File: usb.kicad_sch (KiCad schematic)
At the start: 20 parts, among them J12 USB_A, J3 2169900003, Q1 MMBT3904, U12 STMPS2141STR

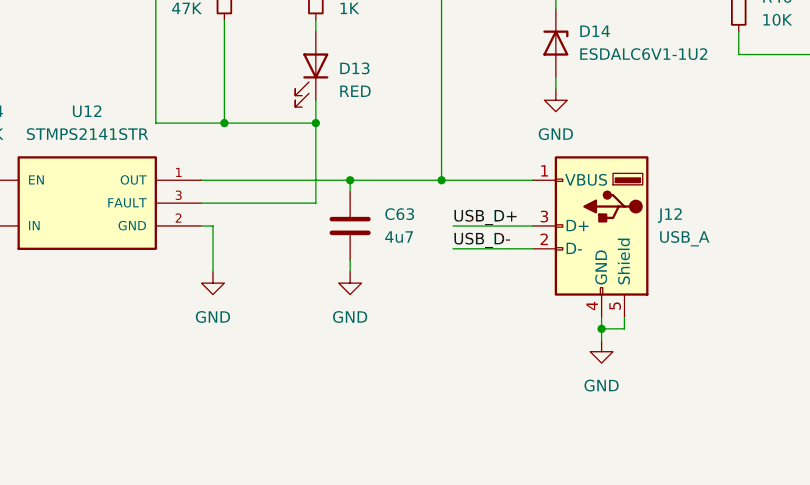
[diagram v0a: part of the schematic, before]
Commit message: First release
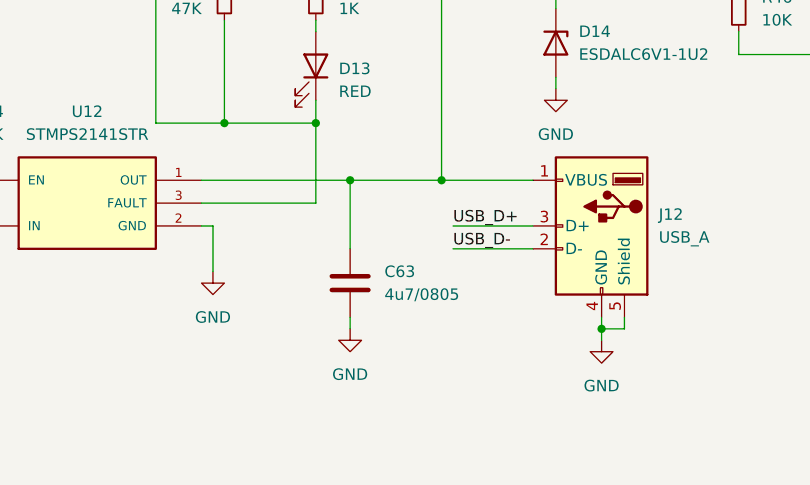
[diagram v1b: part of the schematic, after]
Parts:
- C63: value 4u7 -> 4u7/0805
- D14: JLCPCB Part # (none) -> C1974498; now left out of the parts list
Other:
- moved on the sheet: C63
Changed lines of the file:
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@@
 	(wire
 		(pts
-			(xy 109.22 121.92) (xy 109.22 123.19)
+			(xy 109.22 128.27) (xy 109.22 129.54)
 		)
 		(stroke
@@
 	(wire
 		(pts
-			(xy 109.22 113.03) (xy 109.22 114.3)
+			(xy 109.22 113.03) (xy 109.22 120.65)
 		)
 		(stroke
@@
 	(symbol
 		(lib_id "Device:C")
-		(at 109.22 118.11 0)
+		(at 109.22 124.46 0)
 		(unit 1)
 		(exclude_from_sim no)
@@
 		(fields_autoplaced yes)
 		(property "Reference" "C63"
-			(at 113.03 116.8399 0)
+			(at 113.03 123.1899 0)
 			(effects
 				(font
@@
 			)
 		)
-		(property "Value" "4u7"
-			(at 113.03 119.3799 0)
+		(property "Value" "4u7/0805"
+			(at 113.03 125.7299 0)
 			(effects
 				(font
@@
 		)
 		(property "Footprint" "Capacitor_SMD:C_0805_2012Metric"
-			(at 110.1852 121.92 0)
+			(at 110.1852 128.27 0)
 			(effects
 				(font
@@
 		)
 		(property "Datasheet" "~"
-			(at 109.22 118.11 0)
+			(at 109.22 124.46 0)
 			(effects
 				(font
@@
 		)
 		(property "Description" "Unpolarized capacitor"
-			(at 109.22 118.11 0)
+			(at 109.22 124.46 0)
 			(effects
 				(font
@@
 		)
 		(property "JLCPCB Part #" "C98192"
-			(at 109.22 118.11 0)
+			(at 109.22 124.46 0)
 			(effects
 				(font
@@
 		)
 		(property "Arrow Part Number" ""
-			(at 109.22 118.11 0)
+			(at 109.22 124.46 0)
 			(effects
 				(font
@@
 		)
 		(property "Arrow Price/Stock" ""
-			(at 109.22 118.11 0)
+			(at 109.22 124.46 0)
 			(effects
 				(font
@@
 		)
 		(property "Height" ""
-			(at 109.22 118.11 0)
+			(at 109.22 124.46 0)
 			(effects
 				(font
@@
 		)
 		(property "Manufacturer_Name" ""
-			(at 109.22 118.11 0)
+			(at 109.22 124.46 0)
 			(effects
 				(font
@@
 		)
 		(property "Manufacturer_Part_Number" ""
-			(at 109.22 118.11 0)
+			(at 109.22 124.46 0)
 			(effects
 				(font
@@
 		)
 		(property "Mouser Part Number" ""
-			(at 109.22 118.11 0)
+			(at 109.22 124.46 0)
 			(effects
 				(font
@@
 		)
 		(property "Mouser Price/Stock" ""
-			(at 109.22 118.11 0)
+			(at 109.22 124.46 0)
 			(effects
 				(font
@@
 	(symbol
 		(lib_id "power:GND")
-		(at 109.22 123.19 0)
+		(at 109.22 129.54 0)
 		(unit 1)
 		(exclude_from_sim no)
@@
 		(fields_autoplaced yes)
 		(property "Reference" "#PWR0143"
-			(at 109.22 129.54 0)
+			(at 109.22 135.89 0)
 			(effects
 				(font
@@
 		)
 		(property "Value" "GND"
-			(at 109.22 128.27 0)
+			(at 109.22 134.62 0)
 			(effects
 				(font
@@
 		)
 		(property "Footprint" ""
-			(at 109.22 123.19 0)
+			(at 109.22 129.54 0)
 			(effects
 				(font
@@
 		)
 		(property "Datasheet" ""
-			(at 109.22 123.19 0)
+			(at 109.22 129.54 0)
 			(effects
 				(font
@@
 		)
 		(property "Description" "Power symbol creates a global label with name \"GND\" , ground"
-			(at 109.22 123.19 0)
+			(at 109.22 129.54 0)
 			(effects
 				(font
@@
 		(unit 1)
 		(exclude_from_sim no)
-		(in_bom yes)
+		(in_bom no)
 		(on_board yes)
 		(dnp no)
@@
 			(at 132.08 97.79 0)
 			(effects
+				(font
+					(size 1.27 1.27)
+				)
+				(hide yes)
+			)
+		)
+		(property "JLCPCB Part #" "C1974498"
+			(at 132.08 97.79 0)
+			(effects
